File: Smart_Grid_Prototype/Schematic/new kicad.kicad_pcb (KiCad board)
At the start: 2 copper layers, 144.8 x 116.8 mm, 70 parts, among them J1 EXT_POW, J2 24VAC _LOAD, J3 AC_INPUT, J4 DC_LOAD, J5 POW_SHARE, Q1 BD139, Q2 BD139, Q3 BD139, Q4 BD139, Q5 BD139, Q6 BD139, Q7 BD139, U1 ESP8266, U10 PC817, U11 PC817, U12 PC817, U13 PC817, U14 PC817, U15 PC817, U16 PC817, U2 RELAY_INT, U3 RELAY_PS, U4 PC817, U5 LM7824_TO220, U6 PC817, U7 PC817, U8 LM317_TO-220, U9 PC817

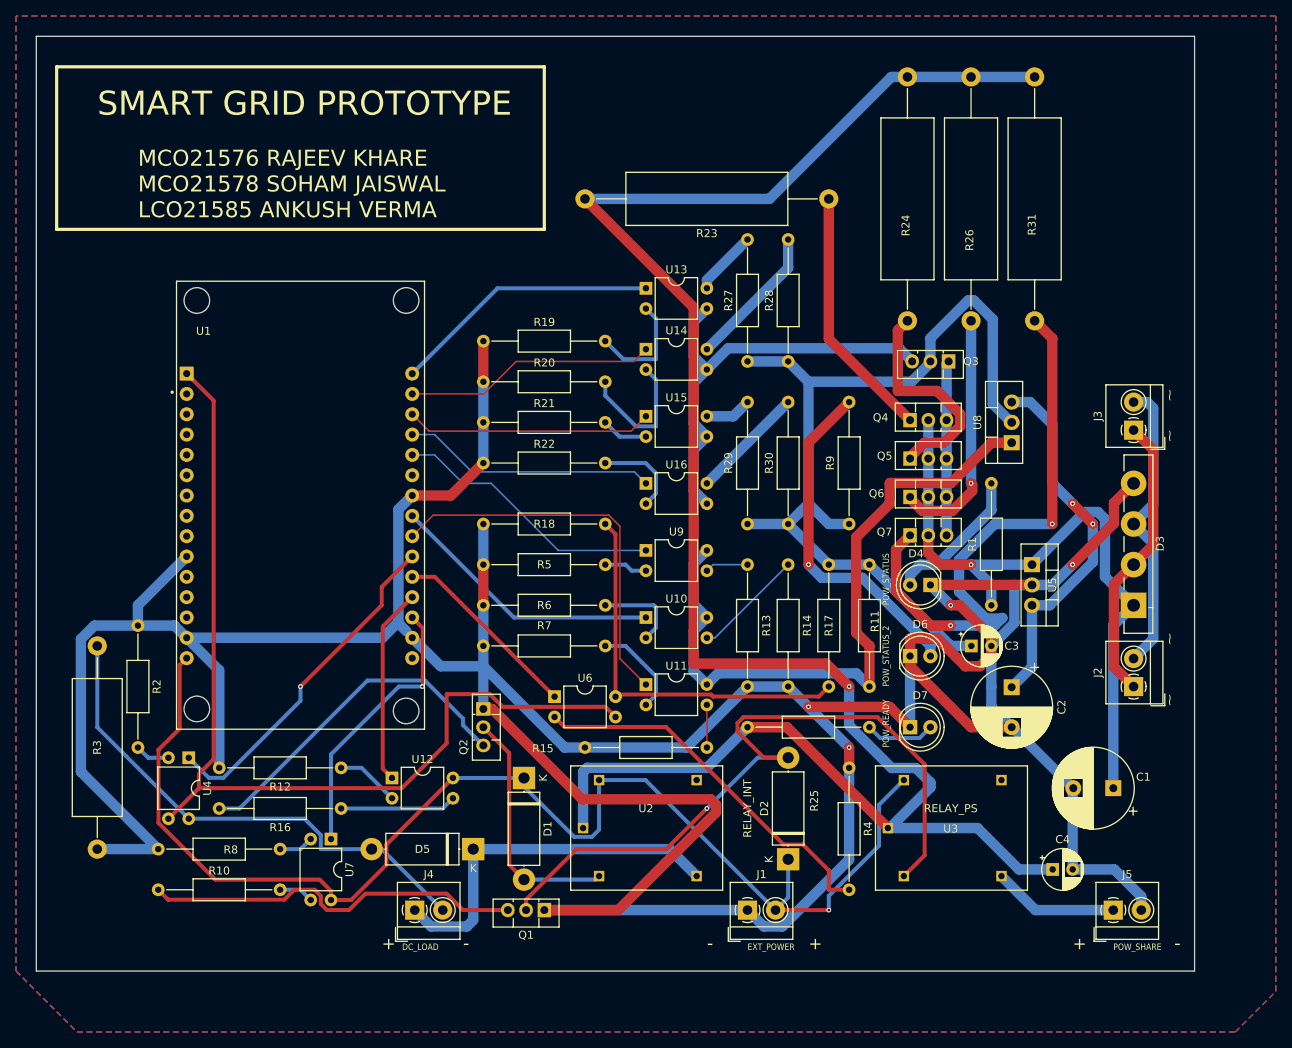
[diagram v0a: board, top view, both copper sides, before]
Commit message: only saved
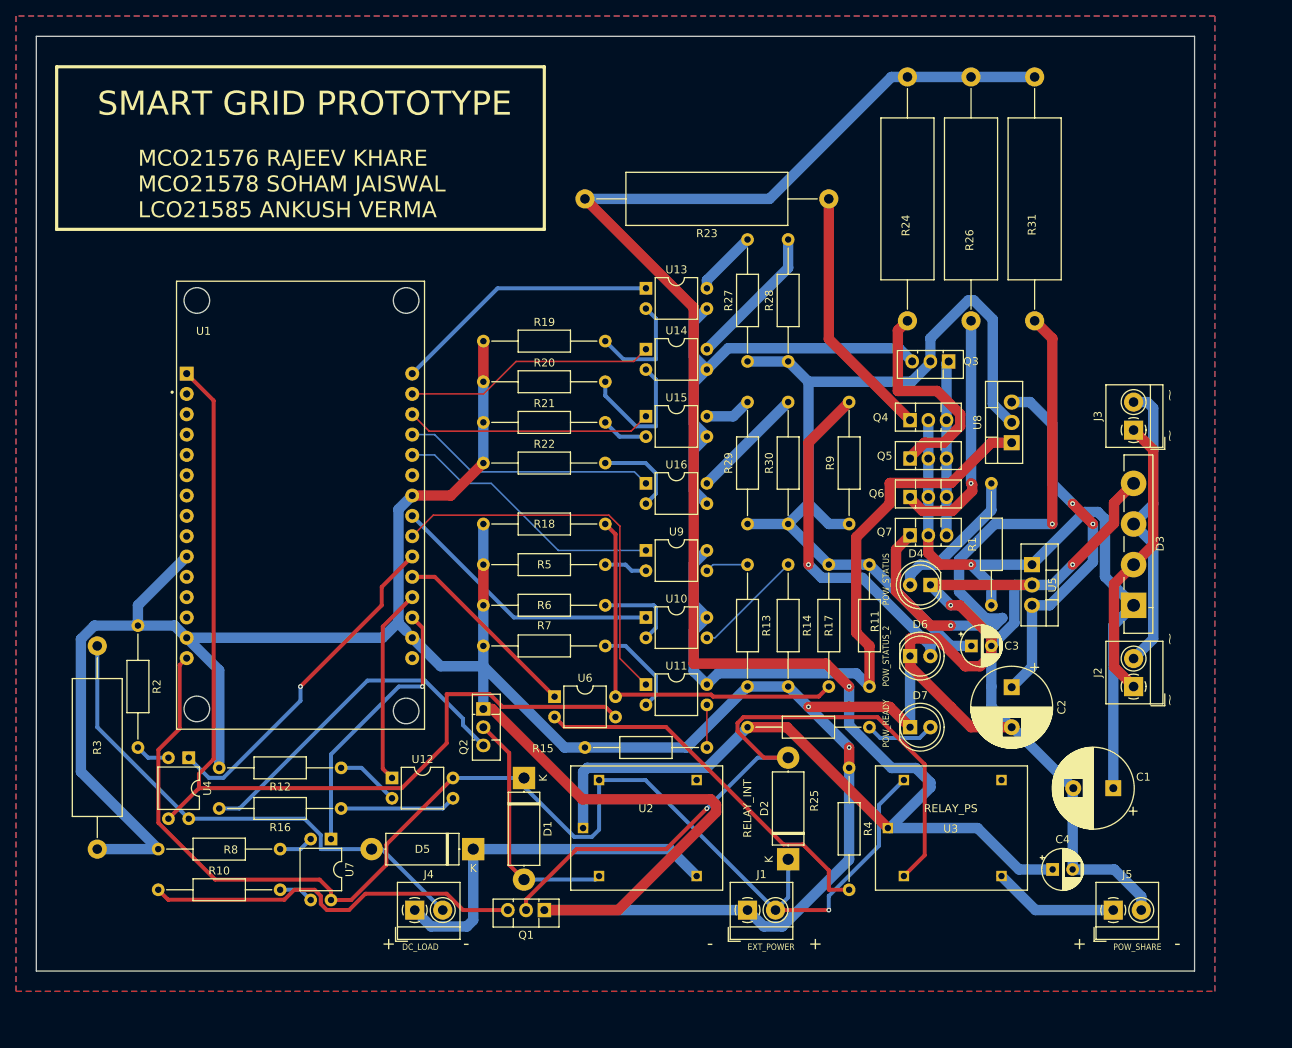
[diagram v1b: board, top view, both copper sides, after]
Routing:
- added copper zone on B.Cu, net GND
- added copper zone on F.Cu, net GND
- removed copper zone on B.Cu, net (none)
- removed copper zone on F.Cu, net (none)
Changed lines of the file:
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@@
 	)
 	(zone
-		(net 0)
-		(net_name "")
+		(net 1)
+		(net_name "GND")
 		(layers "F&B.Cu")
 		(hatch edge 0.5)
@@
 			(thermal_gap 0.5)
 			(thermal_bridge_width 0.5)
-			(island_removal_mode 1)
-			(island_area_min 10)
 		)
 		(polygon
 			(pts
-				(xy 68.58 152.4) (xy 76.2 160.02) (xy 220.98 160.02) (xy 226.06 154.94) (xy 226.06 33.02) (xy 68.58 33.02)
+				(xy 68.58 33.02) (xy 68.58 154.94) (xy 218.44 154.94) (xy 218.44 33.02)
 			)
 		)
